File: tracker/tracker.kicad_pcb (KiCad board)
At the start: 2 copper layers, 40 x 42.5 mm, 22 parts, among them J1 USB_C_Receptacle_PowerOnly_6P, Q1 DMG9926UDM-7, U1 XIAO-ESP32-C6-SMD, U2 LIS3DH, U3 DW01A, U4 INA226AIDGSR, U5 TP4056-42-ESOP8

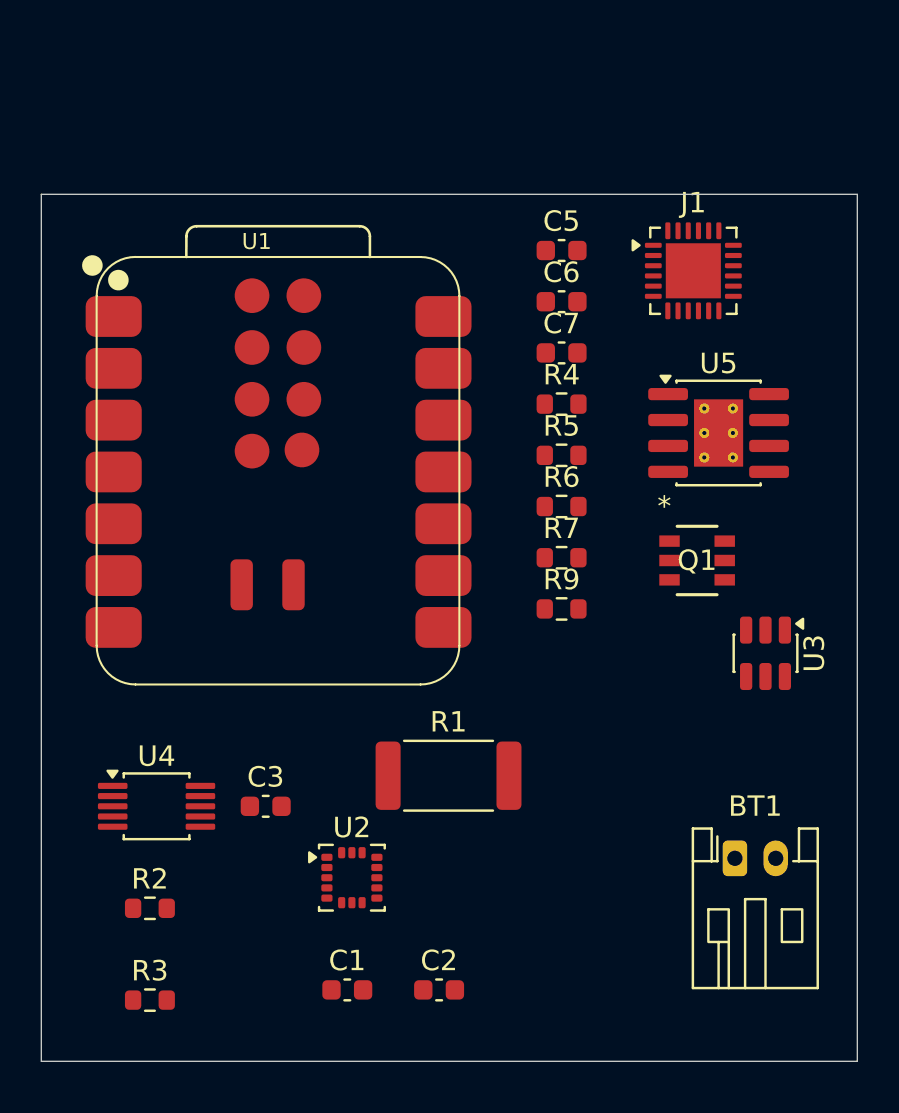
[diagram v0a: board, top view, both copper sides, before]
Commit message: added led's
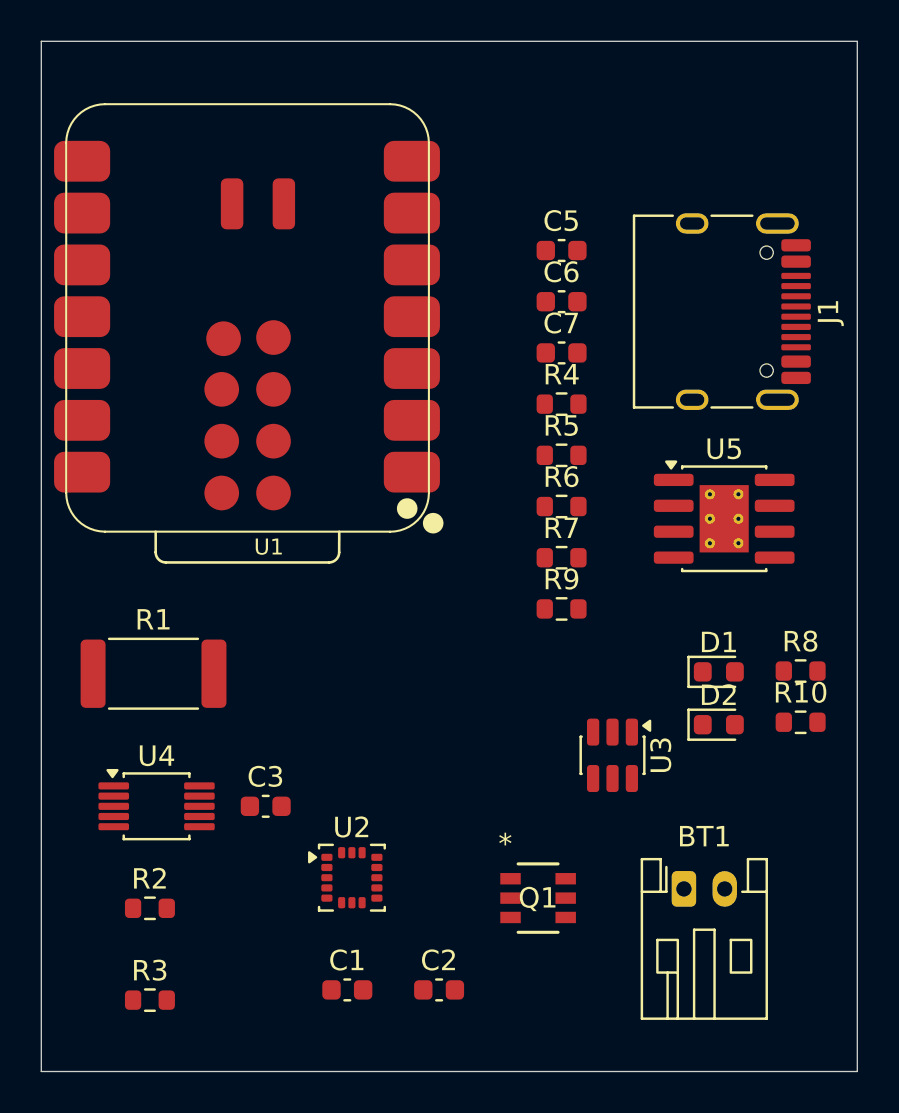
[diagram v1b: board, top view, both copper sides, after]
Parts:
- added D1: LED, LED_SMD:LED_0603_1608Metric, F.Cu at (143.7, 106.9)
- added D2: LED, LED_SMD:LED_0603_1608Metric, F.Cu at (143.7, 109.5)
- added R10: 680, Resistor_SMD:R_0603_1608Metric, F.Cu at (147.7, 109.4)
- added R8: 680, Resistor_SMD:R_0603_1608Metric, F.Cu at (147.7, 106.9)
- J1: footprint Package_DFN_QFN:QFN-24-1EP_4x4mm_P0.5mm_EP2.7x2.7mm -> Connector_USB:USB_C_Receptacle_HRO_TYPE-C-31-M-12
- R4: value 2.4k -> 1.2k
- U4: footprint Package_SO:TSSOP-10_3x3mm_P0.5mm -> Package_SO:MSOP-10_3x3mm_P0.5mm
- moved U1 32.9 mm to (129.5, 79.0), turned to 180 degrees
- moved Q1 18.3 mm to (134.9, 118.0)
- moved R1 15.3 mm to (116.0, 107.0)
- moved U3 9.01 mm to (138.5, 111.0)
- moved U5 4.21 mm to (144.0, 99.4)
- moved BT1 2.92 mm to (142.0, 117.5)
- moved J1 2.23 mm to (143.5, 89.2), turned to -90 degrees
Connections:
- net Net-(U1-VBAT) renamed /Shunt_Output
- U5 pad 6: unconnected-(U5-~{STDBY}-Pad6) -> Net-(D2-K)
- U5 pad 7: unconnected-(U5-~{CHRG}-Pad7) -> Net-(D1-K)
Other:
- board size 40 x 42.5 mm -> 40 x 50.5 mm
